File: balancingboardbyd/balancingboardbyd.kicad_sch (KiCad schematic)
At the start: 74 parts, among them CN1 XT30PW-M, CN2 WJ15EDGRC-3.81-4P, CN3 WJ15EDGRC-3.81-4P, Q1 KMBTA94, Q10 SI2302A-TP, Q11 IRFH5302TRPBF, Q2 SI2302A-TP, Q3 SI2302A-TP, Q4 SI2302A-TP, Q5 SI2302A-TP, Q6 KMBTA94, Q7 IRFH5302TRPBF, Q8 NCE0103Y, Q9 SI2302A-TP, U1 BM3451UNDC-T28A, U2 BM3451UNDC-T28A, U3 XT30PW-F

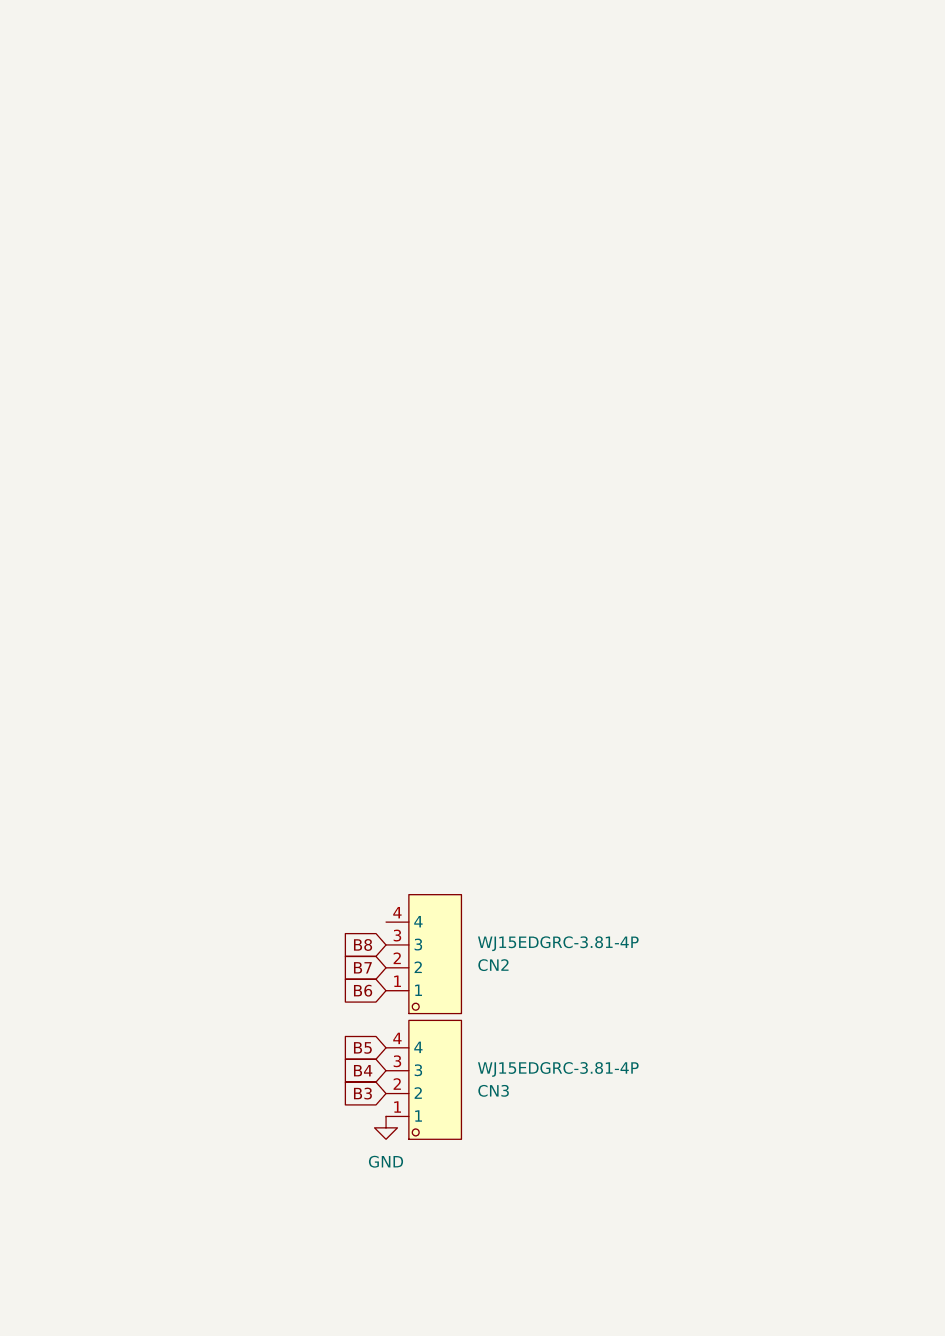
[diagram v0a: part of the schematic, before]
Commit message: next step
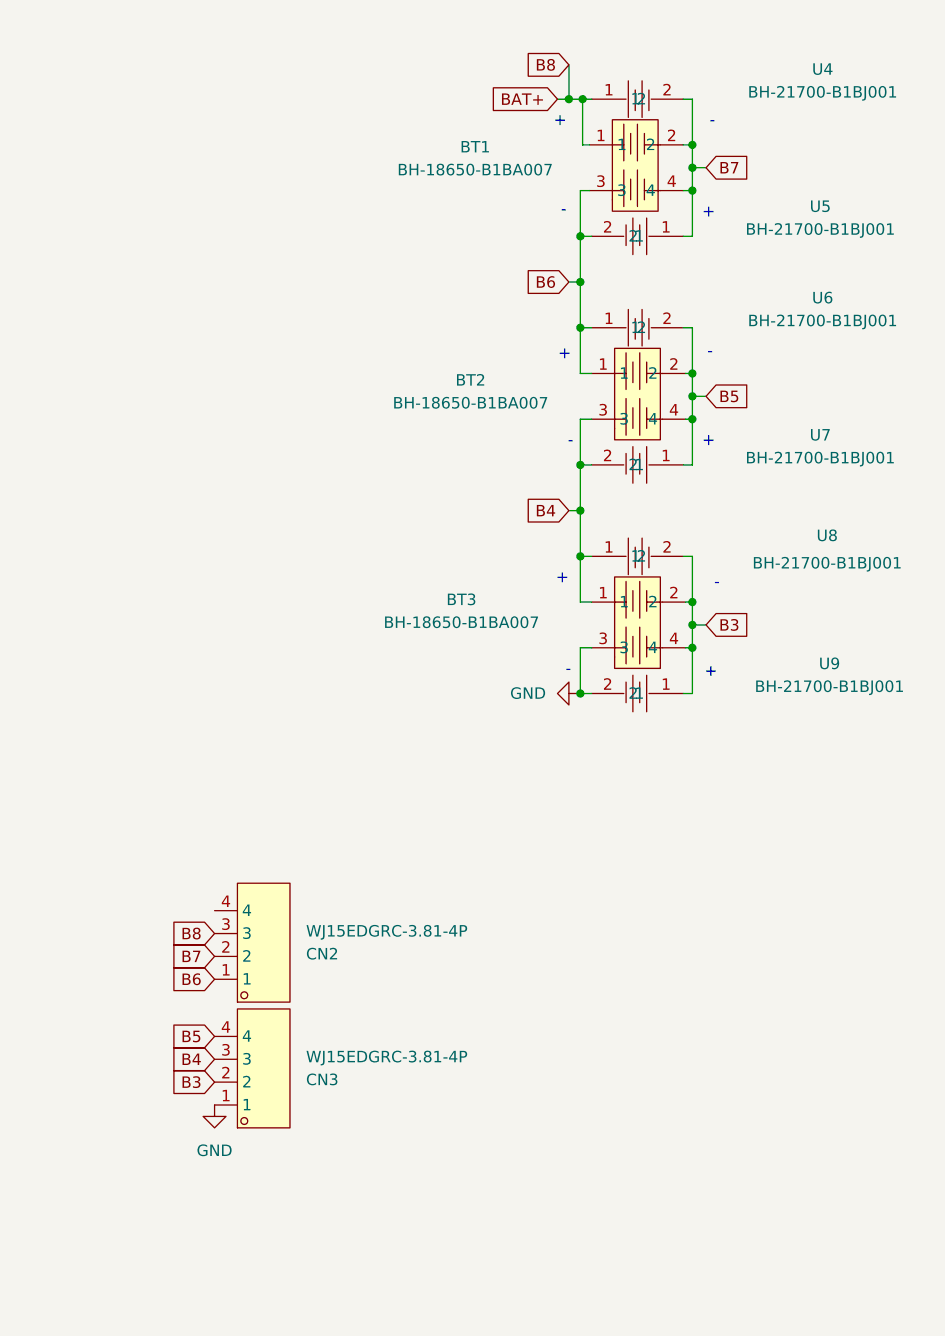
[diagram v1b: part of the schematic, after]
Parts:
- added BT1, BT2, BT3: BH-18650-B1BA007, easyeda2kicad:BAT-SMD_BH-18650-B1BA007, symbol easyeda2kicad:BH-18650-B1BA007
- added U4, U5, U6, U7, U8, U9: BH-21700-B1BJ001, easyeda2kicad:BAT-SMD_L82.5.5-W25-BH-21700-B1BJ001, symbol easyeda2kicad:BH-21700-B1BJ001
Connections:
- net BAT+ is gone; now on net B8: CN1.2 (+), U3.1
- net B3: now also BT3.2, BT3.4, U8.2, U9.1
- net B4: now also BT2.3, BT3.1, U7.2, U8.1
- net B5: now also BT2.2, BT2.4, U6.2, U7.1
- net B6: now also BT1.3, BT2.1, U5.2, U6.1
- net B7: now also BT1.2, BT1.4, U4.2, U5.1
- net B8: now also BT1.1, U4.1
- net GND: now also BT3.3, U9.2
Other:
- note added: "+"
- note added: "-"
- moved on the sheet: CN2, CN3
